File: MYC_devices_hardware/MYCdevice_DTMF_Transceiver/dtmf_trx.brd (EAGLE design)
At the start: 65.4 x 41.6 mm, 33 parts, among them IC1 78L05Z, IC2 MT8880, IC4 MEGA8-P, Q1 20MHz, Q2 3,579545MHz, X1 8-15V, X2 1503_09, X3 1503_09

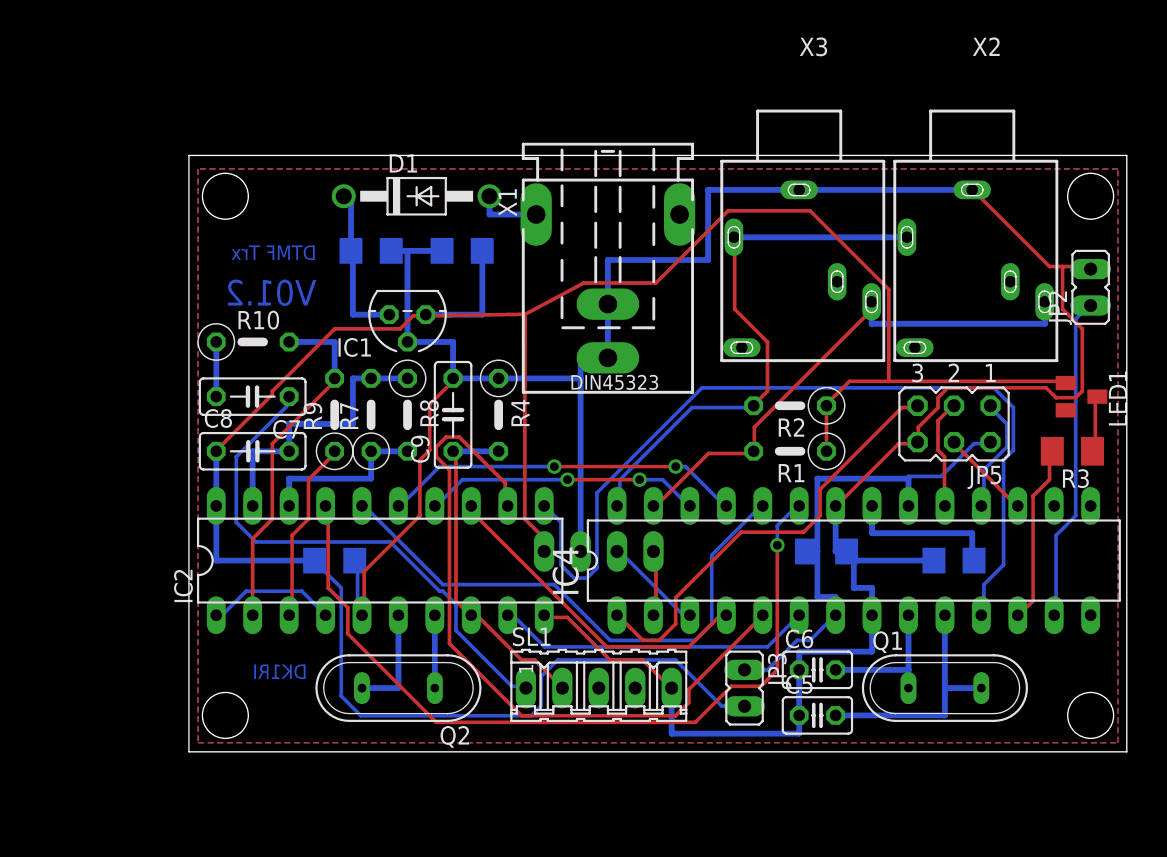
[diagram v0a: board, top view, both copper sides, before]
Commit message: new board
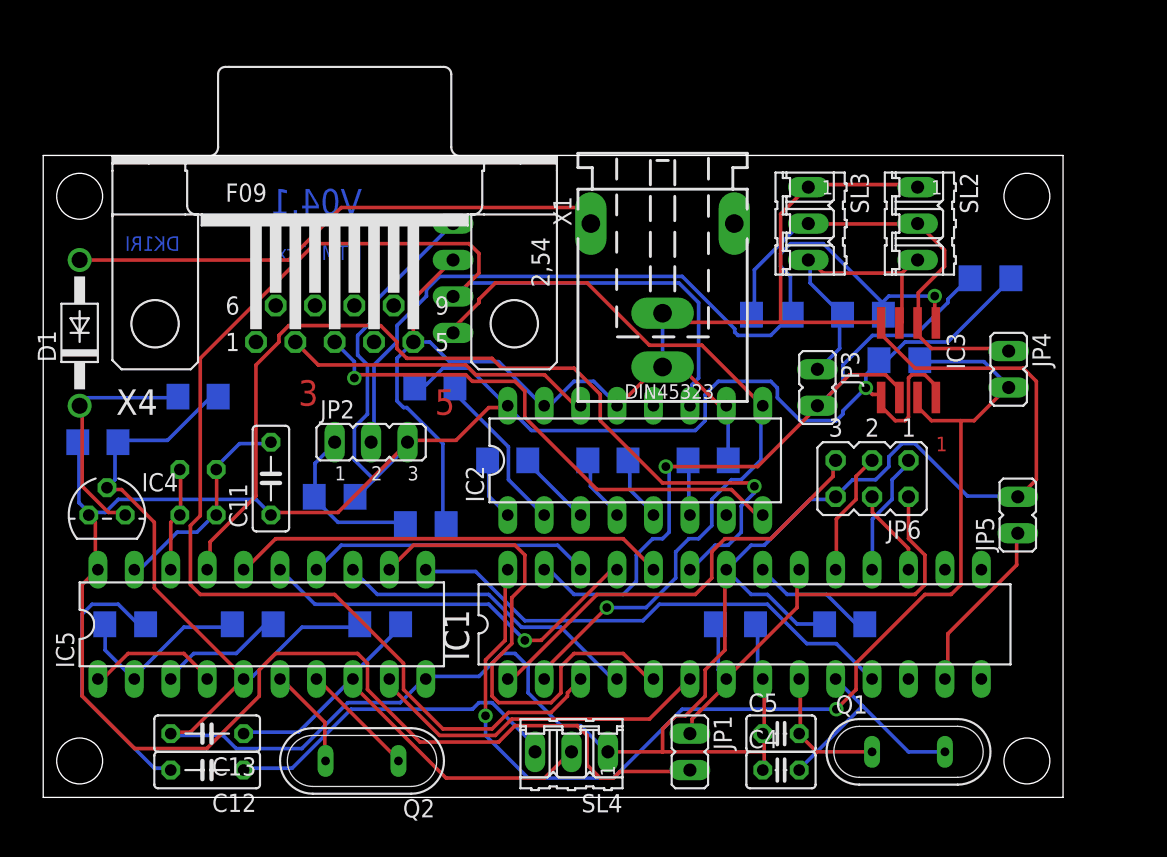
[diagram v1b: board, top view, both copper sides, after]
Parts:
- removed LED1: PL006-WCY01, led:SOT23
- removed SL1: DTMF, con-amp-quick:05P
- removed X2, X3: 1503_09, con-lumberg:1503_09
- added C11, C12: 100n, resistor:C050-025X075
- added C13: 10n, resistor:C050-025X075
- added IC3: PCA9517, PCA9517:SO-08
- added IC5: MT8880, dk1ri:DIL20
- added JP4: SCL, jumper:JP1
- added JP6: ISP, jumper:JP3Q
- added JP7: RS232-USB, jumper:JP4
- added R11: 10k, resistor:R1206
- added R5: 1k, resistor:R1206
- added R6: 1k5, resistor:R1206
- added SL2, SL3: I2c, con-amp-quick:03P
- added SL4: DTMF, con-amp-quick:03P
- added X4: RS232, con-subd:F09H
- C4: value 22uF -> 18pF; device rcl:C1206 -> resistor:C025-025X050
- C6: value 18pF -> 22uF; device resistor:C025-025X050 -> rcl:C1206
- C7, C8: value 100n -> 22uF; device resistor:C050-025X075 -> rcl:C1206
- C9: value 10n -> 22uF; device resistor:C050-025X075 -> rcl:C1206
- IC1: value 78L05Z -> MEGA328; device linear:TO92 -> atmel:DIL28-3
- IC2: value MT8880 -> MAX232; device dk1ri:DIL20 -> maxim:DIL16
- IC4: value MEGA8-P -> 78L05Z; device atmel:DIL28-3 -> linear:TO92
- JP1: value RS232-USB -> Power; device jumper:JP4 -> jumper:JP1
- JP2: value Reset -> 3V/5V; device jumper:JP1 -> jumper:JP2
- JP3: value Power -> SDA
- JP5: value ISP -> Reset; device jumper:JP3Q -> jumper:JP1
- R1, R2: value 4k7 -> see manual; device resistor:0207/5V -> resistor:R1206
- R10, R9: device resistor:0207/5V -> resistor:R1206
- R3: value 4k7 -> see manual; device resistor:M1206 -> resistor:R1206
- R4: value 10k -> see manual; device resistor:0207/5V -> resistor:R1206
- R7, R8: device resistor:0207/5V -> resistor:0309V
- moved IC4 52.2 mm to (18.4, 27.9)
- moved JP2 51.3 mm to (36.8, 33.0)
- moved IC1 31.9 mm to (62.9, 20.3), turned to 0 degrees
- moved C2 28.7 mm to (17.8, 33.0), turned to 180 degrees
- moved C10 28.3 mm to (62.2, 20.3)
- moved R4 28.2 mm to (73.7, 38.7), flipped to the bottom, turned to 180 degrees
- moved C6 26.1 mm to (46.4, 31.8), flipped to the bottom, turned to 180 degrees
- moved D1 25.4 mm to (16.5, 40.6), turned to 90 degrees
- moved C7 25.2 mm to (53.3, 31.8), flipped to the bottom
- moved R10 21.6 mm to (19.7, 20.3), flipped to the bottom
- moved JP3 21.6 mm to (67.9, 36.8)
- moved IC2 19.1 mm to (55.2, 31.8)
- moved C4 18.9 mm to (65.4, 10.2), flipped to the top
- moved C9 18.1 mm to (60.3, 31.8), flipped to the bottom, turned to 180 degrees
- moved R8 16.2 mm to (24.8, 27.9), flipped to the bottom, turned to 0 degrees
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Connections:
- removed net N$1: IC4.12, R3.2
- removed net N$27: IC4.2, JP1.1
- removed net N$35: IC4.3, JP1.2
- removed net N$50: LED1.3, R3.1
- new net N$23: JP2.1, R5.1, R6.2
- new net N$34: C6.2, IC2.3
- new net N$36: C6.1, IC2.1
- new net N$37: IC3.1, JP2.2, R1.1, R2.1
- new net N$38: C7.1, IC2.4
- new net N$39: C7.2, IC2.5
- new net N$40: IC2.8, X4.3
- new net N$41: IC3.3, JP3.1, R1.2, SL2.3, SL3.3
- new net N$42: IC1.28, IC3.7, JP4.2, R4.2
- new net N$43: IC2.14, X4.2
- new net N$45: C9.1, IC2.6
- new net N$46: C8.2, IC2.2
- new net RXD: IC1.2, IC2.9, JP7.1
- new net TXD: IC1.3, IC2.11, JP7.2
- net GND: now also C13.2, C4.1, IC1.22, IC1.8, IC2.13, IC2.15, IC3.4, IC4.2, IC5.10, IC5.5, JP5.2, JP6.6, JP7.3, R11.1, R6.1, SL2.1, SL3.1, SL4.1, X4.5; no longer C4.2, C6.1, IC1.2, IC2.5, IC4.22, IC4.8, JP1.3, JP2.2, JP5.6, R4.1, SL1.5, X2.1, X3.1
- net N$10: now also IC1.25, IC5.15; no longer IC2.15, IC4.25
- net N$11: now also IC1.26, IC5.14; no longer IC2.14, IC4.26
- net N$12: now also IC1.5, IC5.12; no longer IC2.12, IC4.5
- net N$13: now also IC5.6; no longer IC2.6
- net N$14: now also IC5.7; no longer IC2.7
- net N$15: now also IC1.17, JP6.4; no longer IC4.17, JP5.4
- net N$16: now also IC5.1, IC5.4; no longer IC2.1, IC2.4
- net N$17: now also C12.1, SL4.3; no longer C7.1, SL1.1
- net N$18: now also IC1.1, JP6.5; no longer IC4.1, JP5.5
- net N$19: now also C4.2, IC1.10; no longer C5.2, IC4.10
- net N$2: now also IC1.11, IC5.11; no longer IC2.11, IC4.11
- net N$20: now also IC1.18, JP6.1; no longer IC4.18, JP5.1
- net N$21: now also C12.2; no longer C7.2
- net N$22: now also IC3.2, JP4.1, SL2.2, SL3.2; no longer IC4.28, X2.2, X3.2
- net N$24: now also IC5.2; no longer IC2.2
- net N$25: now also C11.2, IC5.19; no longer C8.2, IC2.19
- net N$26: now also C5.2, IC1.9; no longer C6.2, IC4.9
- net N$28: now also IC1.19, JP6.3; no longer IC4.19, JP5.3
- net N$29: now also IC5.3; no longer IC2.3
- net N$3: now also IC1.6, IC5.9; no longer IC2.9, IC4.6
- net N$30: now also C13.1, IC5.8, R11.2, SL4.2; no longer C9.1, IC2.8, R4.2, SL1.2
- net N$31: now also IC5.18; no longer IC2.18
- net N$32: now also C3.1, IC1.21; no longer C4.1, IC4.21
- net N$33: now also IC4.3; no longer IC1.3
- net N$4: now also IC1.4, IC5.13; no longer IC2.13, IC4.4
- net N$5: now also IC1.27, IC3.6, JP3.2, R3.2; no longer IC4.27, R1.2, X2.3, X3.3
- net N$58: now also C10.1, IC1.20, IC1.7, JP1.1, JP6.2; no longer C3.1, IC4.20, IC4.7, JP3.1, JP5.2
- net N$6: now also IC1.13, JP5.1; no longer IC4.13, JP2.1
- net N$8: now also IC1.23, IC5.17; no longer IC2.17, IC4.23
- net N$9: now also IC1.24, IC5.16; no longer IC2.16, IC4.24
- net VDD: now also C11.1, IC2.16, IC3.5, IC3.8, IC4.1, IC5.20, JP1.2, JP2.3, JP7.4, R3.1, R4.1, R5.2; no longer C10.1, IC1.1, IC2.20, JP1.4, JP3.2, LED1.1, R1.1, R2.1
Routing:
- net TXD: track 0.00 -> 102.5 mm
- net N$42: track 0.00 -> 80.1 mm, vias 0 -> 2
- net GND: track 194.3 -> 266.3 mm
- net N$37: track 0.00 -> 61.7 mm, vias 0 -> 1
- net RXD: track 0.00 -> 54.7 mm, vias 0 -> 1
- net N$40: track 0.00 -> 36.8 mm, vias 0 -> 1
- net N$7: track 4.52 -> 37.7 mm
- net VDD: track 166.0 -> 197.3 mm, vias 0 -> 1
- net N$2: track 61.1 -> 35.2 mm
- net N$43: track 0.00 -> 21.8 mm
- net N$41: track 0.00 -> 21.5 mm
- net N$21: track 3.81 -> 19.4 mm
- net N$5: track 37.6 -> 52.1 mm, vias 0 -> 1
- net N$12: track 49.7 -> 36.0 mm
- net N$1: track 12.5 -> 0.00 mm
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- removed copper zone on layer 1, net GND
- removed copper zone on layer 16, net GND
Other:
- board size 65.4 x 41.6 mm -> 71.1 x 44.8 mm
- board text added: "1"
- board text added: "3"
- board text added: "5"
- board text added: "V04.1"
- board text removed: "V01.2"
